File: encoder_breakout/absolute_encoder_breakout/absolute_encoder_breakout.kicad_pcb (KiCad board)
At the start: 2 copper layers, 14.5 x 9.7 mm, 3 parts

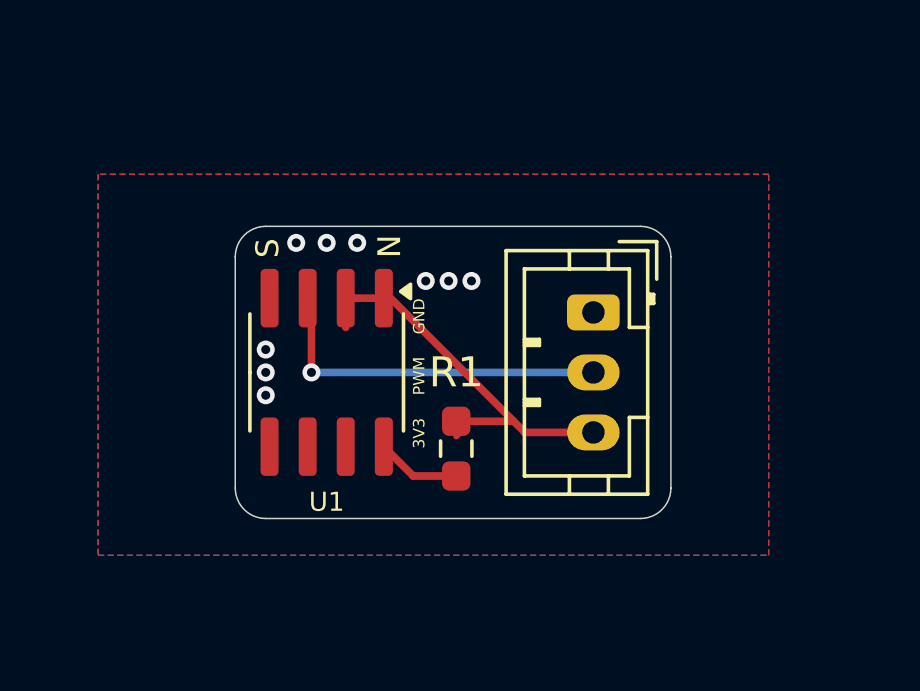
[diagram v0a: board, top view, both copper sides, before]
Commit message: Final Encoder Breakout
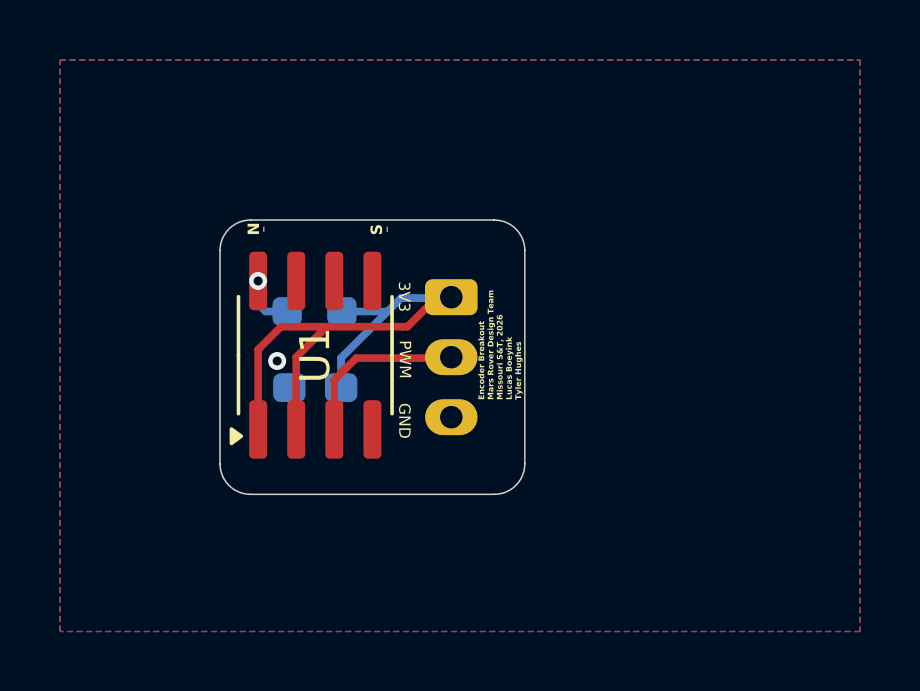
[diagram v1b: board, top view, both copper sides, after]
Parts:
- removed Conn1: Molex_SL_03, Connector_JST:JST_PH_B3B-PH-K_1x03_P2.00mm_Vertical
- added C1: 10uF, Capacitor_SMD:C_0603_1608Metric_Pad1.08x0.95mm_HandSolder, B.Cu at (139.3, 75.7)
- added J1: Conn_01x03_Pin, Connector_JST:JST_PH_S3B-PH-K_1x03_P2.00mm_Horizontal, B.Cu at (143.9, 72.7)
- R1: moved to B.Cu
- moved R1 6.57 mm to (139.3, 73.2), turned to 180 degrees
- moved U1 0.69 mm to (139.3, 74.6), turned to 90 degrees
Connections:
- U1 pad 5: GND -> unconnected-(U1-PGO-Pad5)
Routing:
- net Net-(J1-Pin_2): track 11.9 -> 5.34 mm, vias 1 -> 0
- net Net-(J1-Pin_1): track 13.7 -> 19.7 mm
- net Net-(U1-DIR): track 2.82 -> 1.84 mm, vias 0 -> 1
- net GND: vias 9 -> 1
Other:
- board size 14.5 x 9.7 mm -> 10.2 x 9.1 mm
- board text added: "_"
